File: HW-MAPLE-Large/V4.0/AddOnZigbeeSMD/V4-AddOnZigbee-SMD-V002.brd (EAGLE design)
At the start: 33 x 17 mm, 5 parts

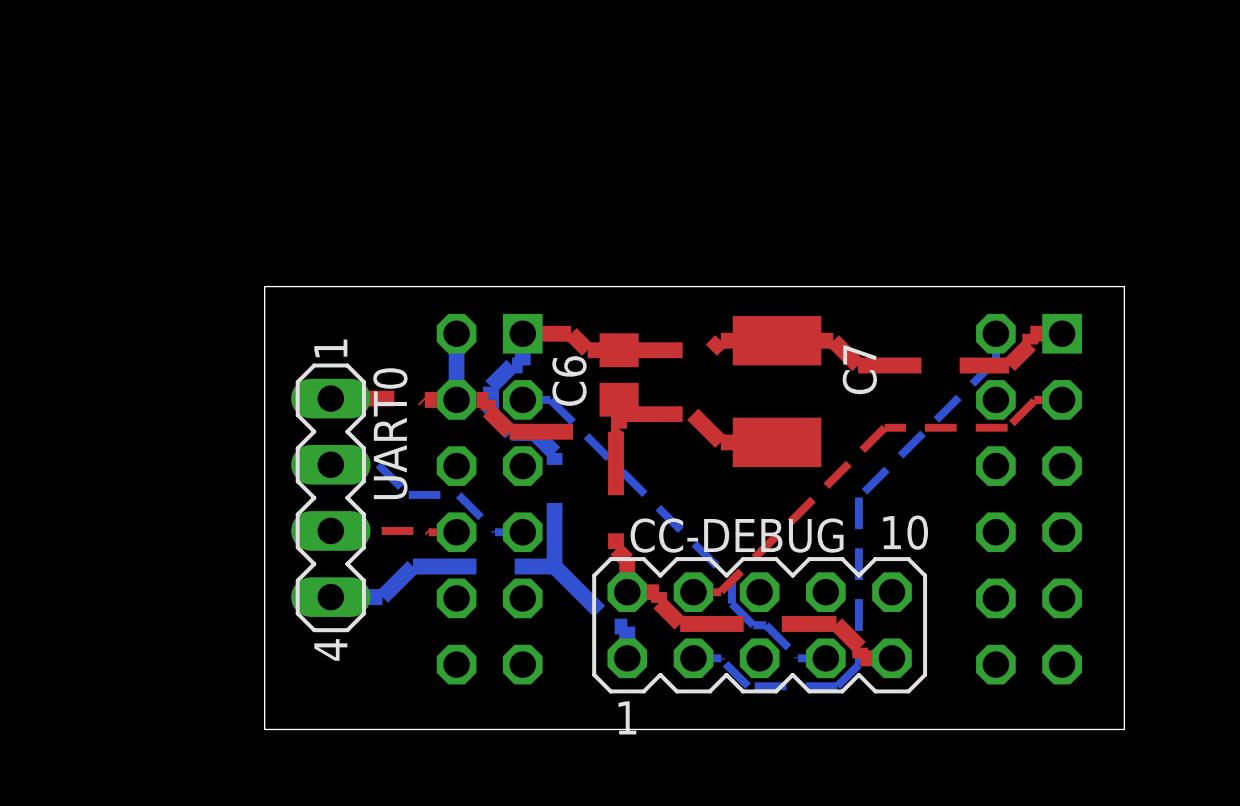
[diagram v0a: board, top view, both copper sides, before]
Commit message: V4 Test
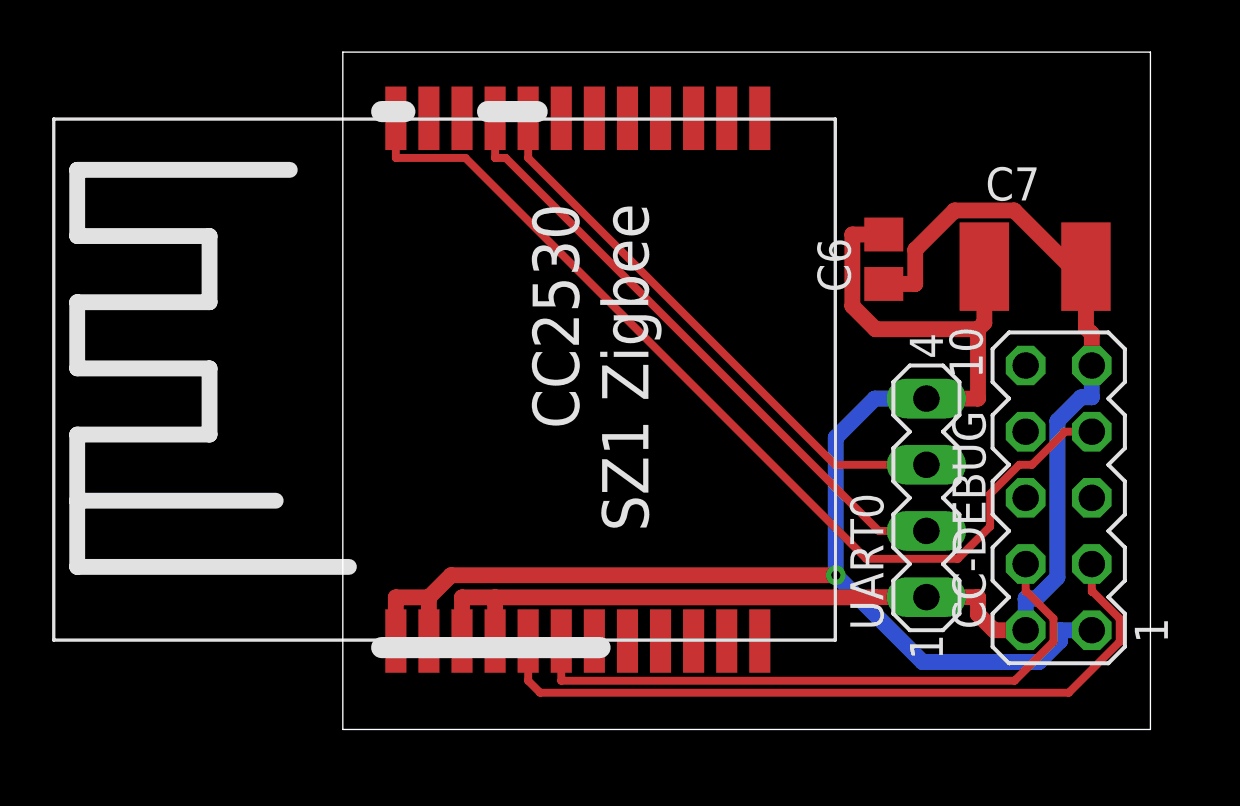
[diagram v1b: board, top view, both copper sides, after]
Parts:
- removed U$3: CC2530_MODULE, Martin-Communication-V4:CC2530_DIL
- added U$1: CC2530, zigbee:SZ1ZIGBEE-SMD
- moved UART0 22.9 mm to (25.4, 8.89), turned to 90 degrees
- moved CC-DEBUG 12.5 mm to (30.5, 8.89), turned to 90 degrees
- moved C6 11.1 mm to (23.8, 18.1)
- moved C7 11.0 mm to (29.6, 17.8), turned to 0 degrees
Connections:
- new net BT: U$1.P$6
- net DC: now also U$1.P$8; no longer U$3.P2_2
- net DD: now also U$1.P$7; no longer U$3.P2_1
- net GND: now also U$1.P$11, U$1.P$12; no longer U$3.GND, U$3.GND2
- net RST: now also U$1.P$24; no longer U$3.RST
- net RX0: now also U$1.P$20; no longer U$3.P0_3\U_TX
- net TX0: now also U$1.P$21; no longer U$3.P0_2\U_RX
- net VCC: now also U$1.P$10, U$1.P$9; no longer U$3.VCC, U$3.VCC2
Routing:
- net RST: track 16.3 -> 37.4 mm
- net RX0: track 4.85 -> 21.7 mm
- net TX0: track 8.46 -> 24.0 mm
- net VCC: track 40.1 -> 52.8 mm
- net GND: track 47.5 -> 58.2 mm, vias 0 -> 1
- net DD: track 17.3 -> 24.5 mm
- net DC: track 22.1 -> 28.7 mm
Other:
- board size 33 x 17 mm -> 31 x 26 mm
